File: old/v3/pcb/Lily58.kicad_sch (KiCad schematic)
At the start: 110 parts, among them P4 OLED, SW1 SW_PUSH, SW10 SW_PUSH, SW11 SW_PUSH, SW12 SW_PUSH, SW13 SW_PUSH, SW14 SW_PUSH, SW15 SW_PUSH, SW16 SW_PUSH, SW17 SW_PUSH, SW18 SW_PUSH, SW19 SW_PUSH, SW2 SW_PUSH, SW20 SW_PUSH, SW21 SW_PUSH, SW22 SW_PUSH, SW23 SW_PUSH, SW24 SW_PUSH, SW25 Rotary_Encoder_Switch, SW26 SW_PUSH, SW27 SW_PUSH, SW28 SW_PUSH, SW29 SW_PUSH, SW3 SW_PUSH, SW4 SW_PUSH, SW5 SW_PUSH, SW6 SW_PUSH, SW7 SW_PUSH, SW8 SW_PUSH, SW9 SW_PUSH, U1 NiceNano

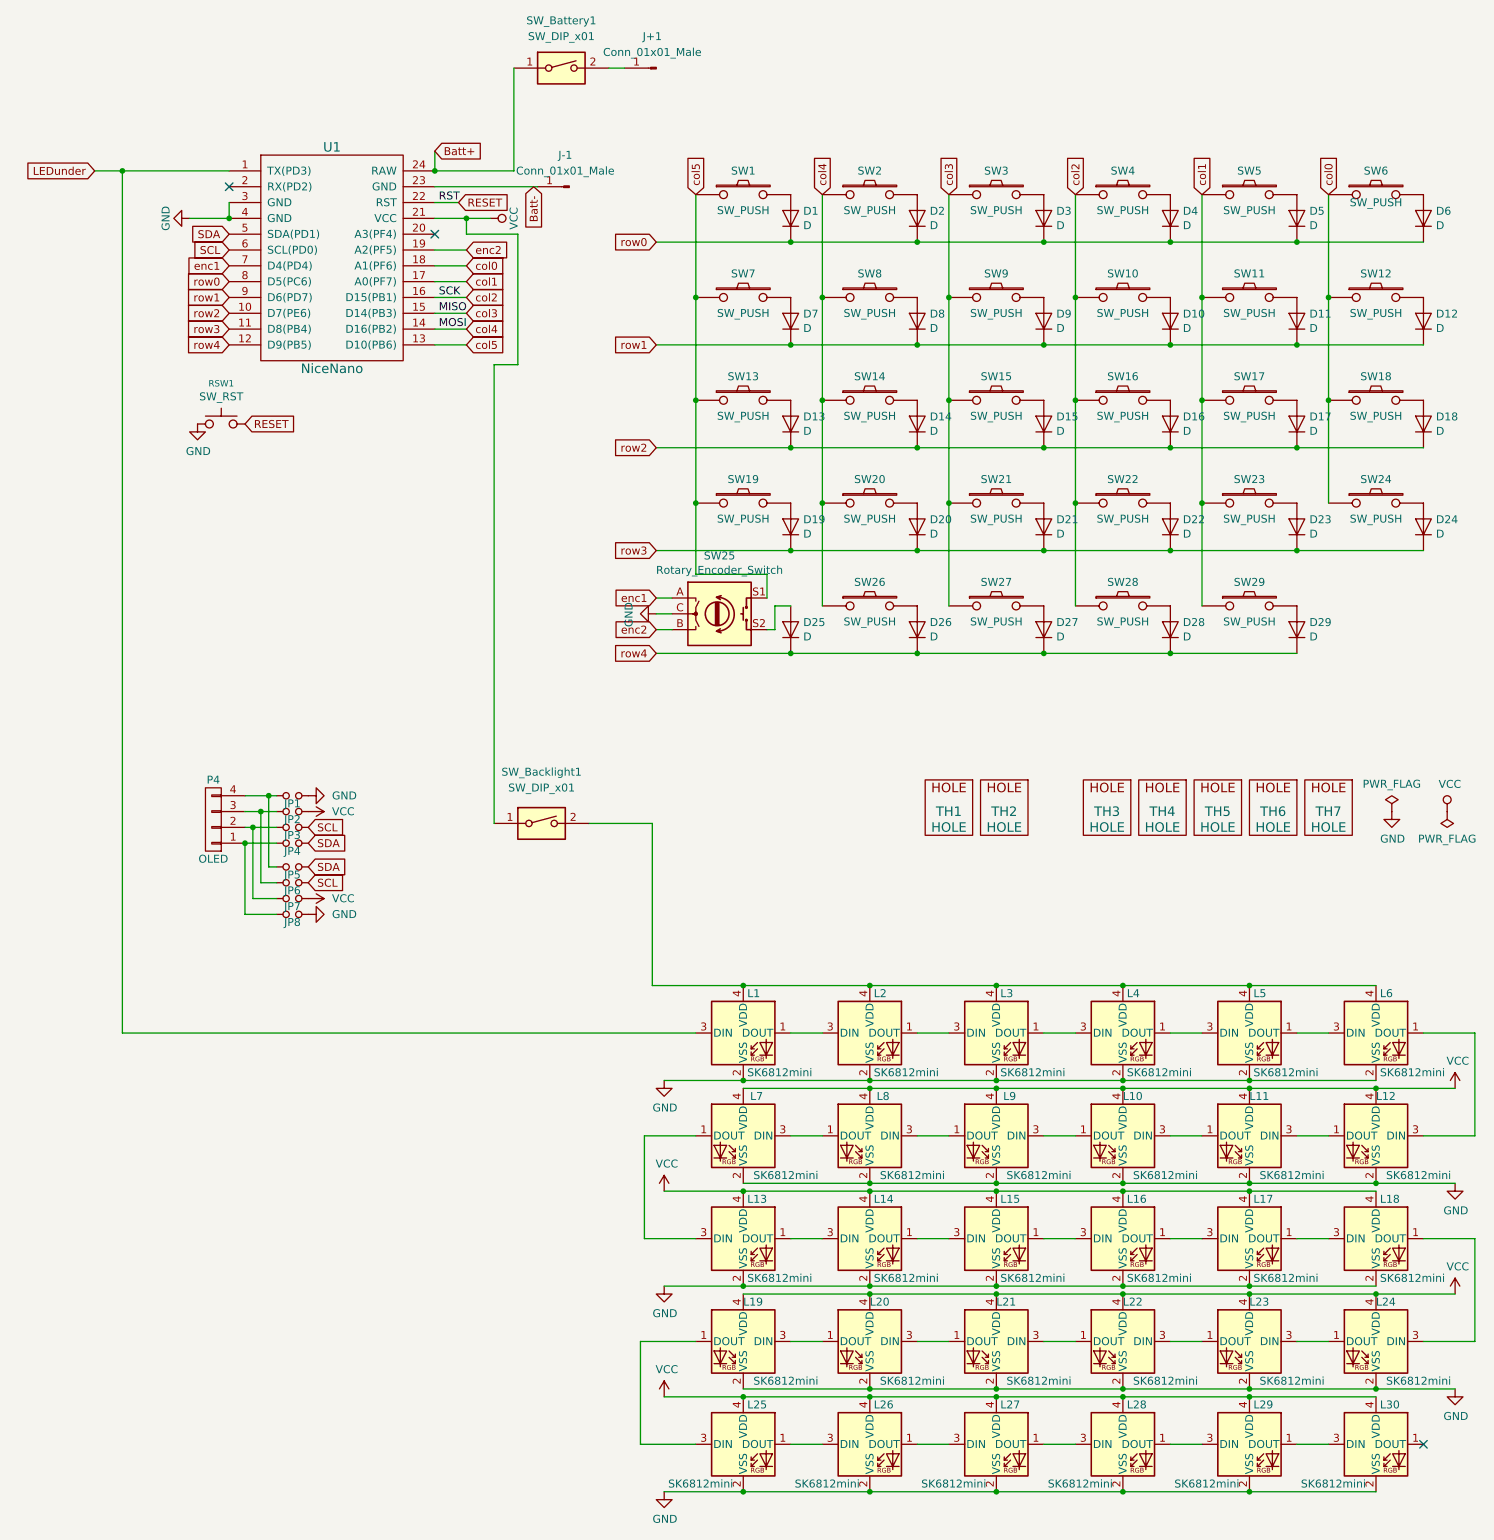
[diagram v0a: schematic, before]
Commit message: Updates to files and layout
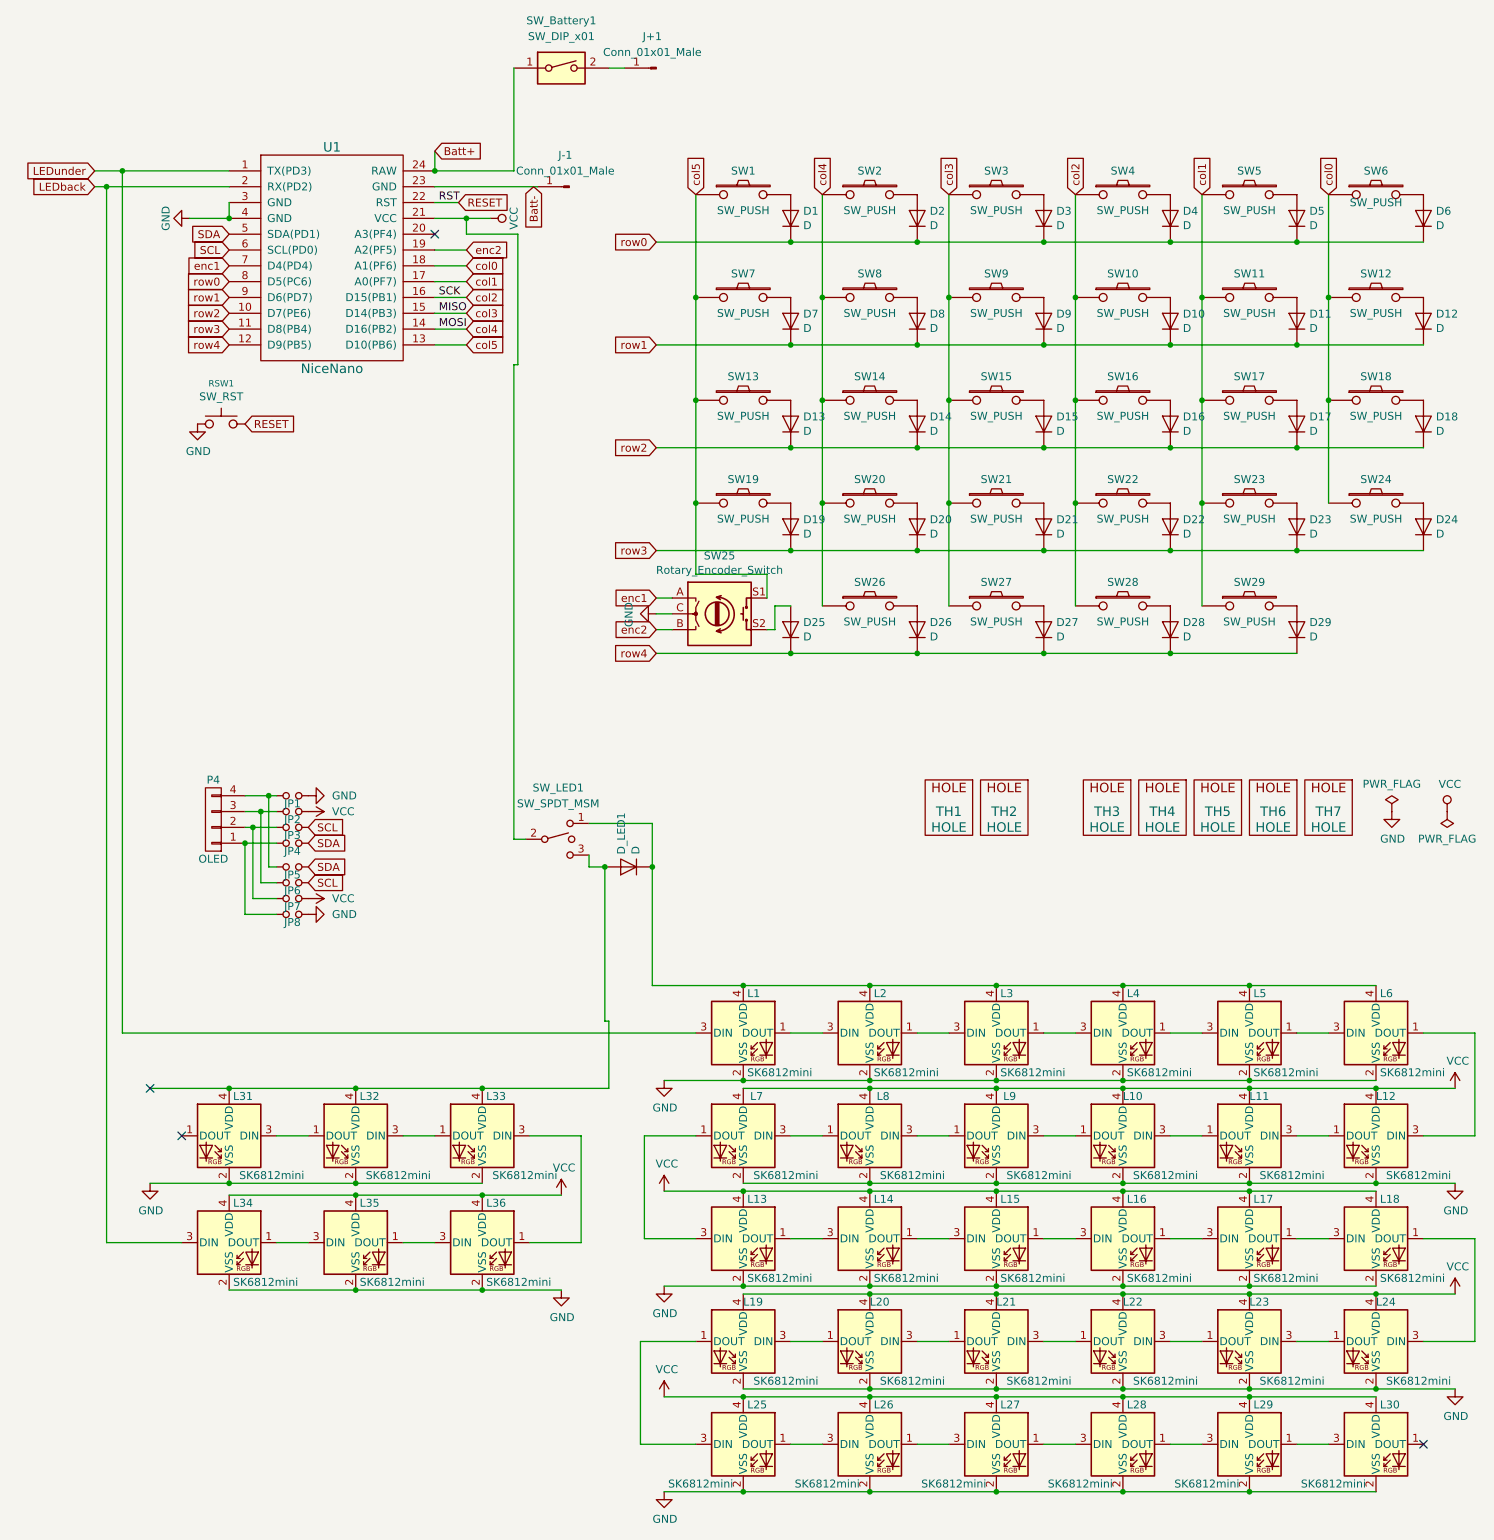
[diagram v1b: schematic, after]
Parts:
- removed SW_Backlight1: SW_DIP_x01, Button_Switch_THT:SW_CuK_OS102011MA1QN1_SPDT_Angled, symbol Switch:SW_DIP_x01
- added D_LED1: D, Diode_THT:D_A-405_P7.62mm_Horizontal, symbol Lily58-rescue:D-Lily58-cache
- added L31, L32, L33, L34, L35, L36: SK6812mini, LED_SMD:LED_SK6812MINI_PLCC4_3.5x3.5mm_P1.75mm, symbol LED:SK6812MINI
- added SW_LED1: SW_SPDT_MSM, AS13AH-KiCad:AS13AH, symbol Switch:SW_SPDT_MSM
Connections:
- net GND: now also L31.2 (VSS), L32.2 (VSS), L33.2 (VSS), L34.2 (VSS), L35.2 (VSS), L36.2 (VSS)
- net VCC: now also L34.4 (VDD), L35.4 (VDD), L36.4 (VDD), SW_LED1.2
- net LEDback: now reaches U1.2 (RX(PD2))
- net LEDback: now also L34.3 (DIN)
- net at L1.4 (VDD), L2.4 (VDD), L3.4 (VDD)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: now also D_LED1.1 (K), SW_LED1.1
- new net: L31.3 (DIN), L32.1 (DOUT)
- new net: D_LED1.2 (A), L31.4 (VDD), L32.4 (VDD), L33.4 (VDD), SW_LED1.3
- new net: L32.3 (DIN), L33.1 (DOUT)
- new net: L33.3 (DIN), L36.1 (DOUT)
- new net: L35.1 (DOUT), L36.3 (DIN)
- new net: L34.1 (DOUT), L35.3 (DIN)
- no-connect marks 3 -> 4
